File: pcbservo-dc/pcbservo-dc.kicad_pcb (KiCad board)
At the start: 4 copper layers, 86 parts, among them IC1 NC7WZ241K8X, IC2 NC7WZ241K8X, IC3 NC7WZ241K8X, J1 Conn_01x02, J10 Conn_01x03, J12 Conn_01x02, J13 Conn_01x02, J14 R-78B5.0-2.0, J2 Conn_01x02, J3 BU33SD5WG-TR, J4 Conn_01x03, J5 Conn_01x03, J7 Conn_ST_STDC14, J8 Conn_01x03, SW1 SW_Nidec_CAS-120A1, SW2 SW_Nidec_CAS-120A1, SW3 SW_Nidec_CAS-120A1, SW4 SW_Nidec_CAS-120A1, SW5 SW_Nidec_CAS-120A1, SW6 SW_Nidec_CAS-120A1, U7 STM32H573RITx

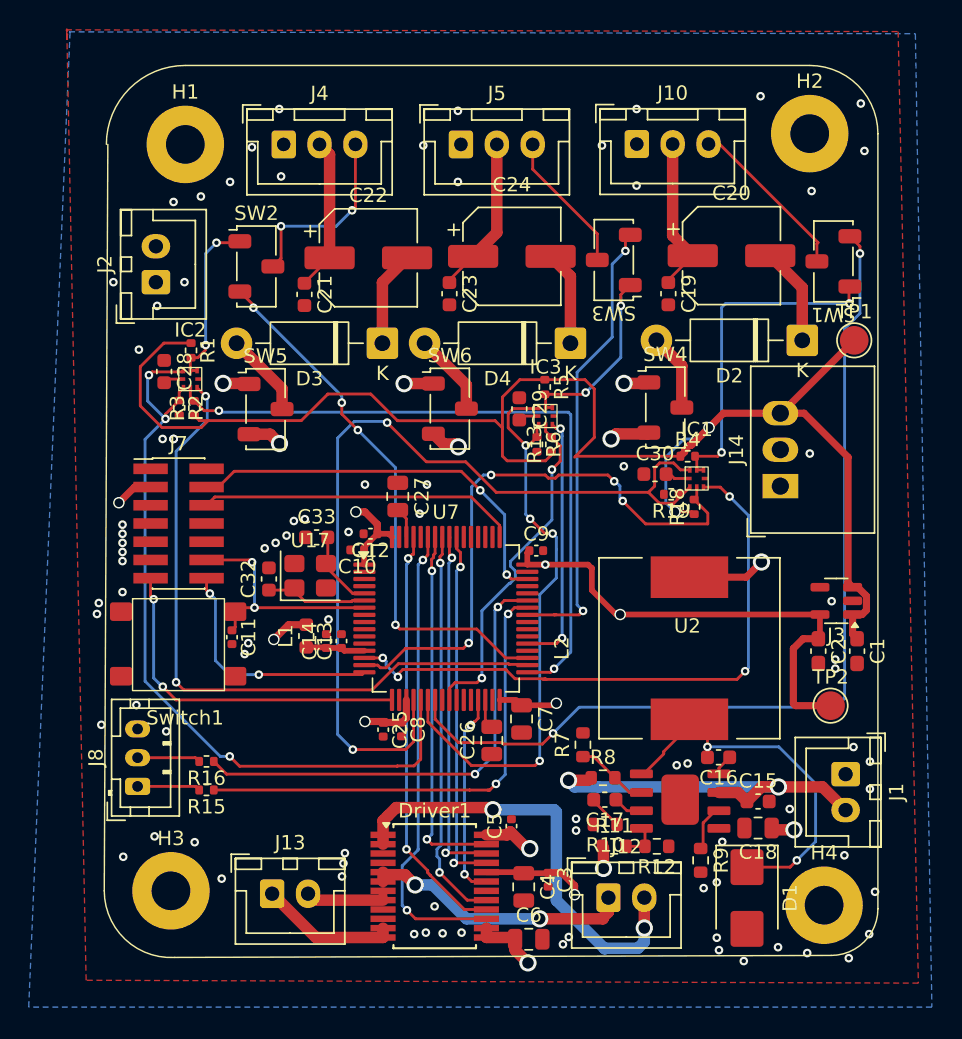
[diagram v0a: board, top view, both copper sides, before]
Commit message: résolution des erreurs
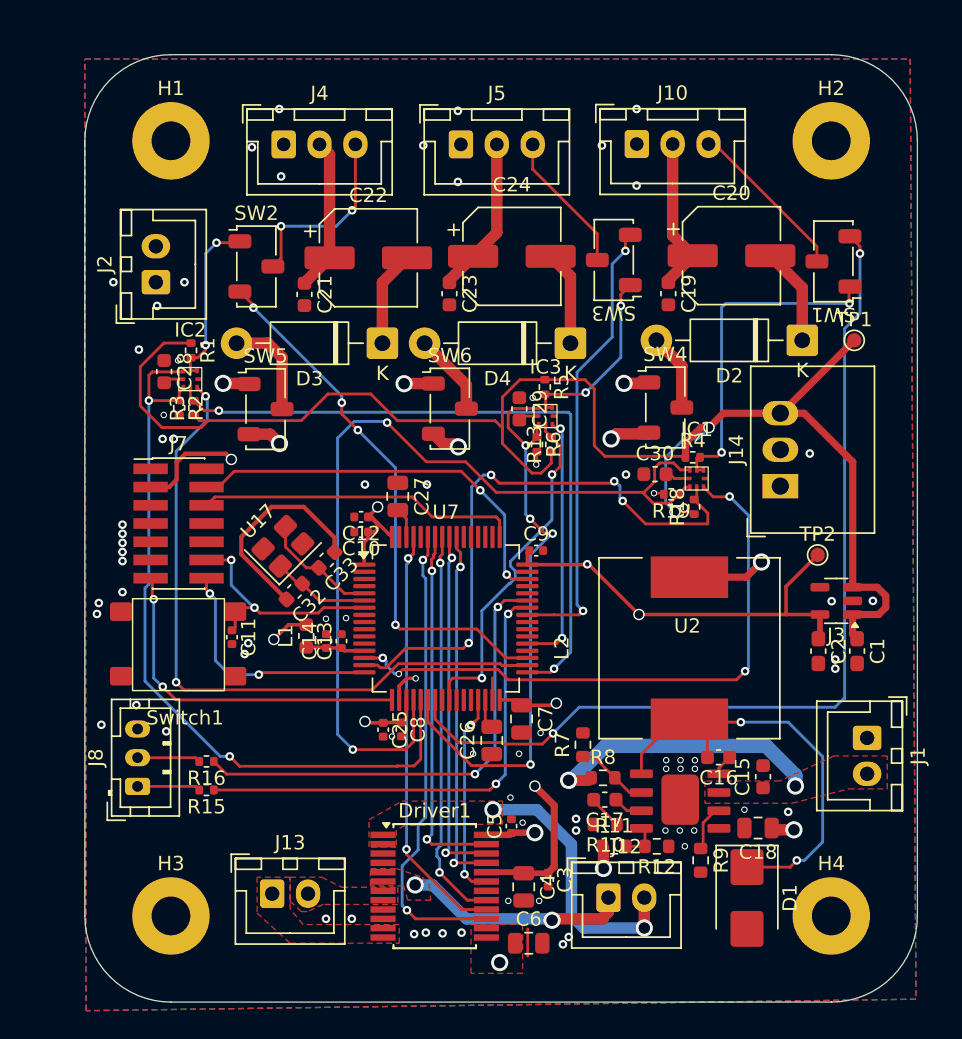
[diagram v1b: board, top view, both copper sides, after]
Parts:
- TP1, TP2: footprint TestPoint:TestPoint_Pad_D2.0mm -> TestPoint:TestPoint_Pad_D1.0mm
- moved TP2 10.5 mm to (215.1, 72.8)
- moved J1 2.94 mm to (218.5, 85.6)
- moved U17 2.80 mm to (177.8, 72.2), turned to 45 degrees
- moved C32 1.98 mm to (178.6, 75.4), turned to -135 degrees
- moved C15 1.76 mm to (211.2, 88.3), turned to 90 degrees
- moved H3 1.75 mm to (170.0, 98.0)
- moved C33 1.72 mm to (180.8, 73.2), turned to -135 degrees
- moved H2 1.58 mm to (216.0, 44.0)
- moved C12 1.34 mm to (183.2, 70.2)
- moved C10 1.28 mm to (183.2, 71.2)
- moved H1 1.03 mm to (170.0, 44.0)
- moved H4 0.90 mm to (216.0, 98.0)
- moved R4 0.36 mm to (206.3, 66.0)
- moved C6 0.28 mm to (194.9, 99.9)
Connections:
- J14 pad 1: +6V -> +25V
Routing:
- net +6V: track 142.6 -> 19.4 mm
- net +3.3V: track 170.9 -> 76.2 mm
- net +?V: track 49.3 -> 5.63 mm
- net GND: track 0.00 -> 22.3 mm, vias 85 -> 75
- net AO1: track 31.2 -> 19.0 mm
- net BO1: track 9.64 -> 0.00 mm
- net +25V: track 26.5 -> 20.0 mm
- net BO2: track 6.01 -> 0.00 mm
- net /regulateur de tension/SW: track 25.8 -> 31.2 mm
- net AO2: track 18.7 -> 15.8 mm
- net Osc_IN: track 5.52 -> 8.26 mm
- net +5V: track 108.9 -> 110.2 mm
- net Alim_servo2: track 5.90 -> 7.18 mm
- net TX2_Enable_5V: track 53.9 -> 53.2 mm, vias 3 -> 2
- net DXL_PWR3: track 13.7 -> 13.1 mm
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- added copper zone on F.Cu, net +25V
- added copper zone on In2.Cu, net +25V
- added copper zone on F.Cu, net +6V
- added copper zone on F.Cu, net AO1
- added copper zone on F.Cu, net AO2
- added copper zone on F.Cu, net BO1
- added copper zone on F.Cu, net BO2
- added copper zone on B.Cu, net GND
- added copper zone on F.Cu, net GND
- removed copper zone on B.Cu, net (none)
- removed copper zone on F.Cu, net (none)
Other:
- board outline added: 58 x 66 mm
